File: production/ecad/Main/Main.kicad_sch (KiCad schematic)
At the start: 1 part, among them J1 61204021621

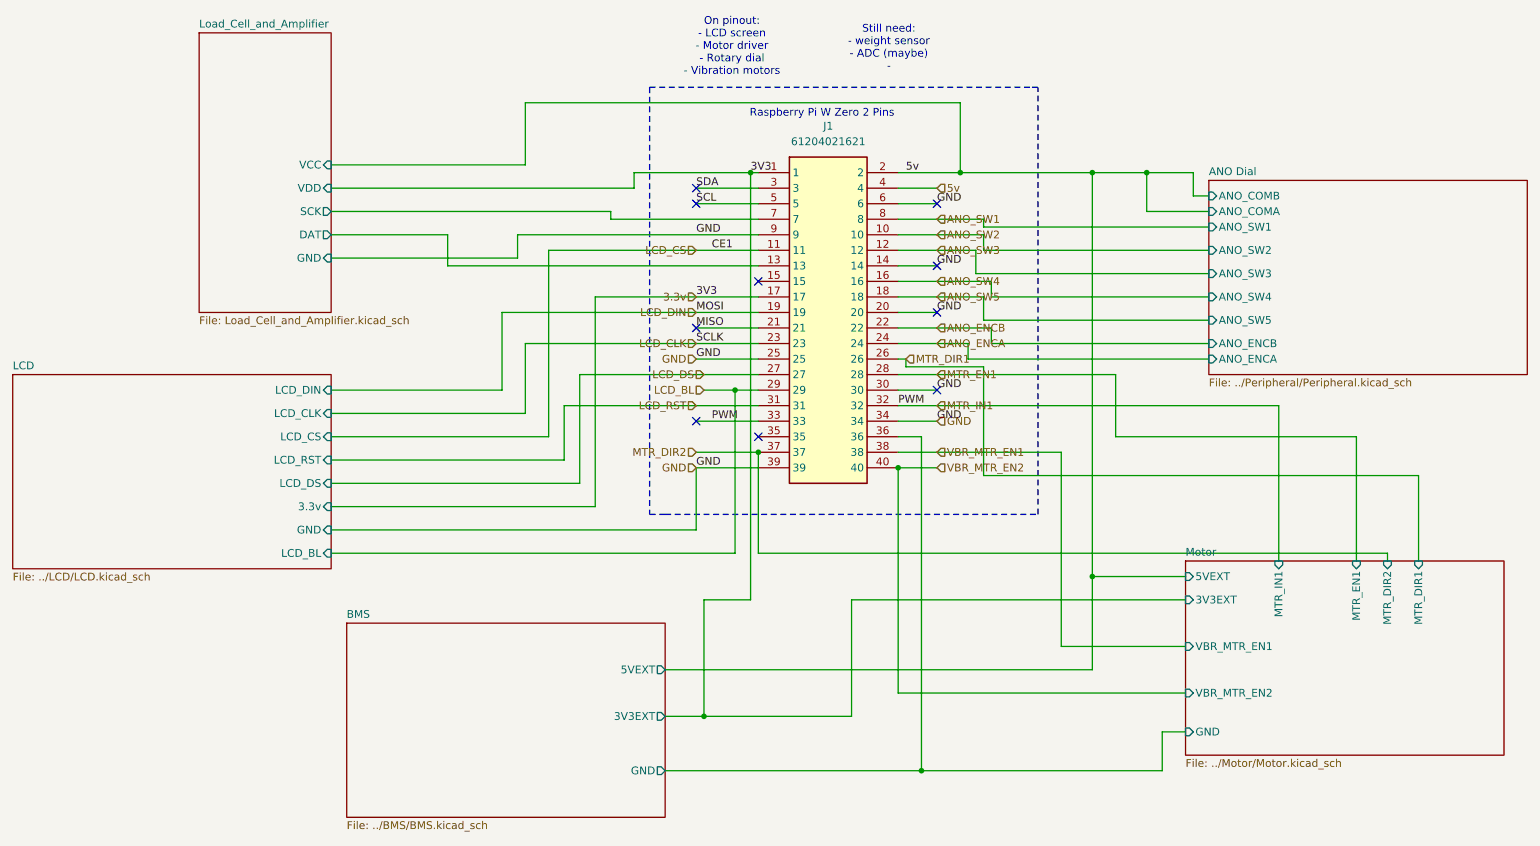
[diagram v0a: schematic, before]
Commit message: feedback
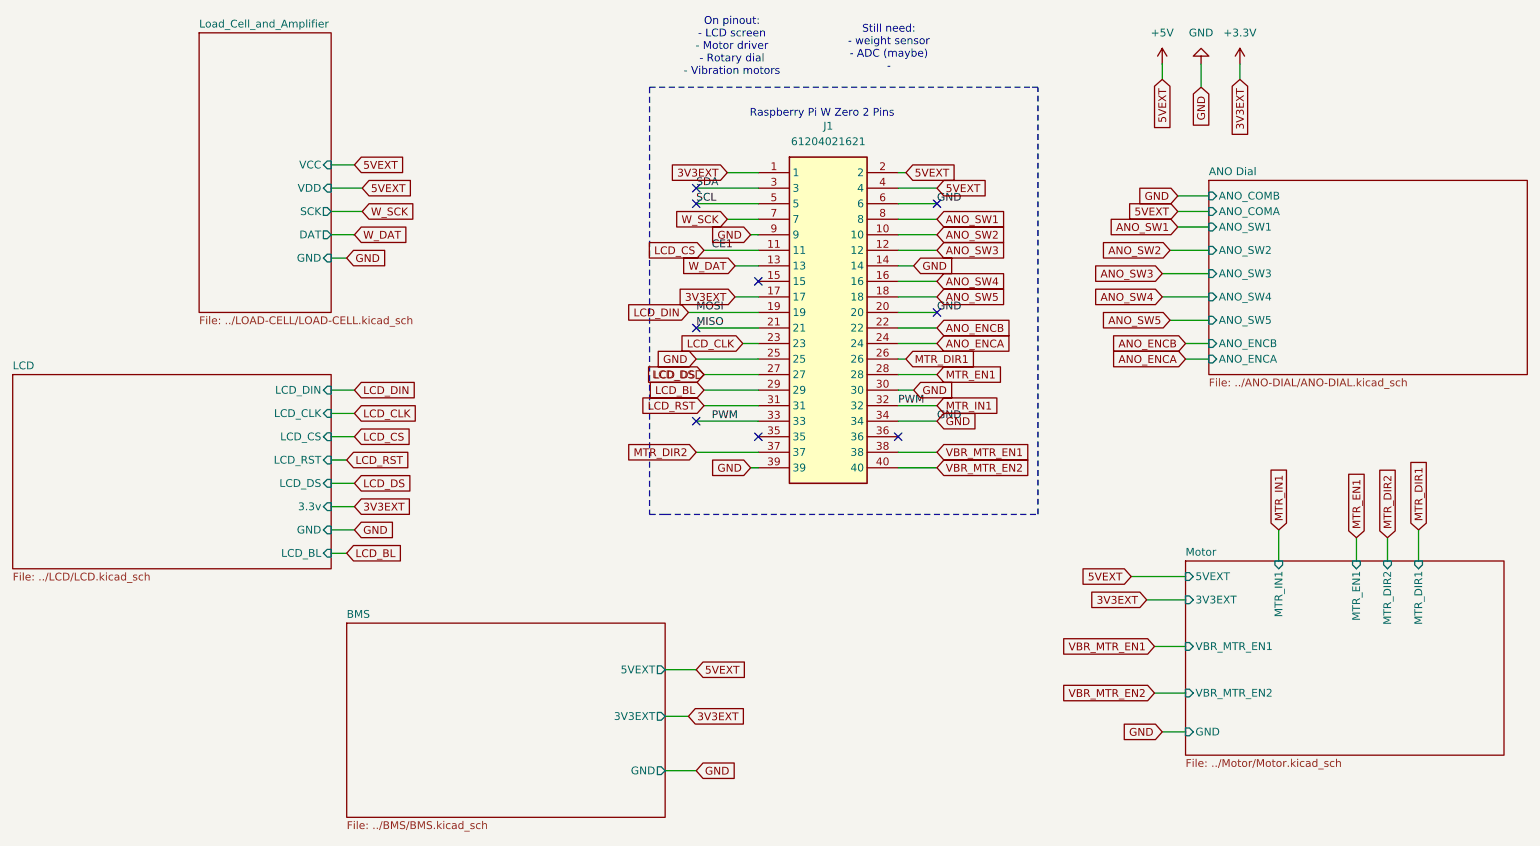
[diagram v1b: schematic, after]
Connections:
- net 3.3v renamed +3.3V
- net 5v renamed +5V
- net BMS/GND: no longer names the net of J1.36
- net Load_Cell_and_Amplifier/DAT renamed W_DAT
- net Load_Cell_and_Amplifier/SCK renamed W_SCK
- no-connect marks 10 -> 9
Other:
- sheet ANO Dial: file ../Peripheral/Peripheral.kicad_sch -> ../ANO-DIAL/ANO-DIAL.kicad_sch
- sheet Load_Cell_and_Amplifier: file Load_Cell_and_Amplifier.kicad_sch -> ../LOAD-CELL/LOAD-CELL.kicad_sch
